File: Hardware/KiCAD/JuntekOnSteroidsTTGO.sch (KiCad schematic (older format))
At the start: 33 parts, among them J1 To PSU host board, J11 patch, J12 patch, J2 To PSU host board, J21 patch, J22 patch, J30 Expansion1, J4 ESP32-TFT, J5 ESP32-TFT, J6 feedback, J61 patch, J7 I2C

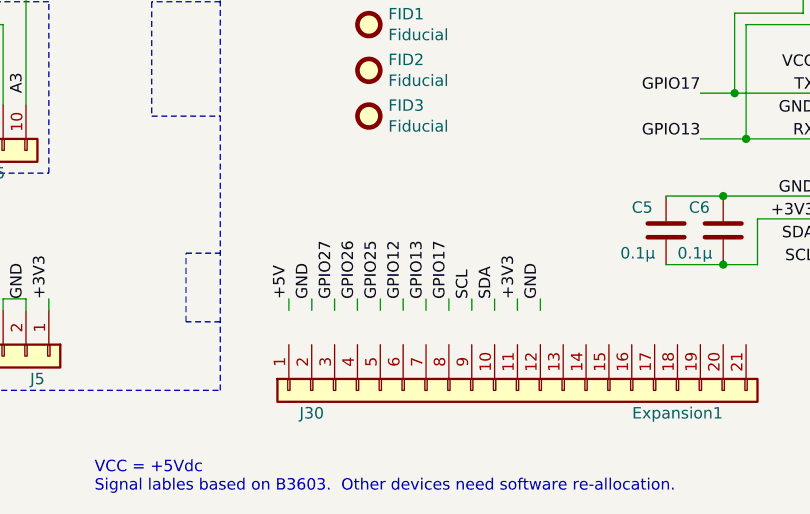
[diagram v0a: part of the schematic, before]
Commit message: routed
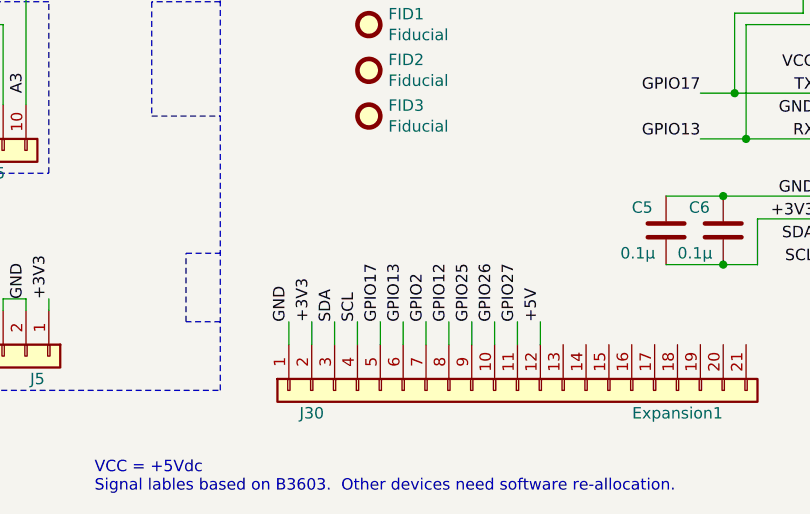
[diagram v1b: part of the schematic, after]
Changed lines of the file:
@@
 Sheet 1 1
 Title "Drok/Juntek-on-steroids"
-Date "2021-08-19"
-Rev "2.3"
+Date "2021-08-21"
+Rev "2.4"
 Comp ""
 Comment1 ""
@@
 	9450 4000 9850 4000
 Connection ~ 9450 4000
-Text Label 9150 5500 1    50   ~ 0
+Text Label 8450 5600 1    50   ~ 0
 SDA
-Text Label 9050 5500 1    50   ~ 0
+Text Label 8550 5600 1    50   ~ 0
 SCL
-Text Label 8850 5500 1    50   ~ 0
+Text Label 8750 5600 1    50   ~ 0
 GPIO13
-Text Label 8950 5500 1    50   ~ 0
+Text Label 8650 5600 1    50   ~ 0
 GPIO17
-Text Label 9350 5500 1    50   ~ 0
-GND
-Text Label 8350 5500 1    50   ~ 0
+Text Label 8250 5600 1    50   ~ 0
 GND
 Text Label 2200 3500 0    50   ~ 0
@@
 Text Label 1750 3900 2    50   ~ 0
 Vset
-Text Label 8750 5500 1    50   ~ 0
+Text Label 8950 5600 1    50   ~ 0
 GPIO12
-Text Label 8650 5500 1    50   ~ 0
+Text Label 9050 5600 1    50   ~ 0
 GPIO25
-Text Label 8550 5500 1    50   ~ 0
+Text Label 9150 5600 1    50   ~ 0
 GPIO26
-Text Label 8450 5500 1    50   ~ 0
+Text Label 9250 5600 1    50   ~ 0
 GPIO27
-Text Label 9250 5500 1    50   ~ 0
+Text Label 8350 5600 1    50   ~ 0
 +3V3
-Text Label 8250 5500 1    50   ~ 0
+Text Label 9350 5600 1    50   ~ 0
 +5V
 Wire Wire Line
@@
 Text Label 1750 3000 2    50   ~ 0
 IloadSense
-Wire Wire Line
-	9350 5500 9350 5550
-Wire Wire Line
-	9250 5550 9250 5500
-Wire Wire Line
-	9150 5500 9150 5550
-Wire Wire Line
-	9050 5550 9050 5500
-Wire Wire Line
-	8950 5500 8950 5550
-Wire Wire Line
-	8850 5550 8850 5500
-Wire Wire Line
-	8750 5500 8750 5550
-Wire Wire Line
-	8650 5550 8650 5500
-Wire Wire Line
-	8550 5500 8550 5550
-Wire Wire Line
-	8450 5550 8450 5500
-Wire Wire Line
-	8350 5500 8350 5550
-Wire Wire Line
-	8250 5550 8250 5500
 $Comp
 L Device:R R14
@@
 	1    0    0    -1
 $EndComp
+Text Label 8850 5600 1    50   ~ 0
+GPIO2
+Wire Wire Line
+	8250 5600 8250 5700
+Wire Wire Line
+	8350 5600 8350 5700
+Wire Wire Line
+	8450 5600 8450 5700
+Wire Wire Line
+	8550 5600 8550 5700
+Wire Wire Line
+	8650 5600 8650 5700
+Wire Wire Line
+	8750 5600 8750 5700
+Wire Wire Line
+	8850 5600 8850 5700
+Wire Wire Line
+	8950 5600 8950 5700
+Wire Wire Line
+	9050 5600 9050 5700
+Wire Wire Line
+	9150 5600 9150 5700
+Wire Wire Line
+	9250 5600 9250 5700
+Wire Wire Line
+	9350 5600 9350 5700
 $EndSCHEMATC
